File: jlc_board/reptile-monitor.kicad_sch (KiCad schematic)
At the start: 28 parts, among them J1 AudioJack4_SwitchR1, J2 AudioJack4_SwitchR1, J3 PWR CONN, J4 UART, J5 I2C, SW1 RESET, SW2 BOOT, U1 AP2112M-3.3, U2 TCA4307DGKR

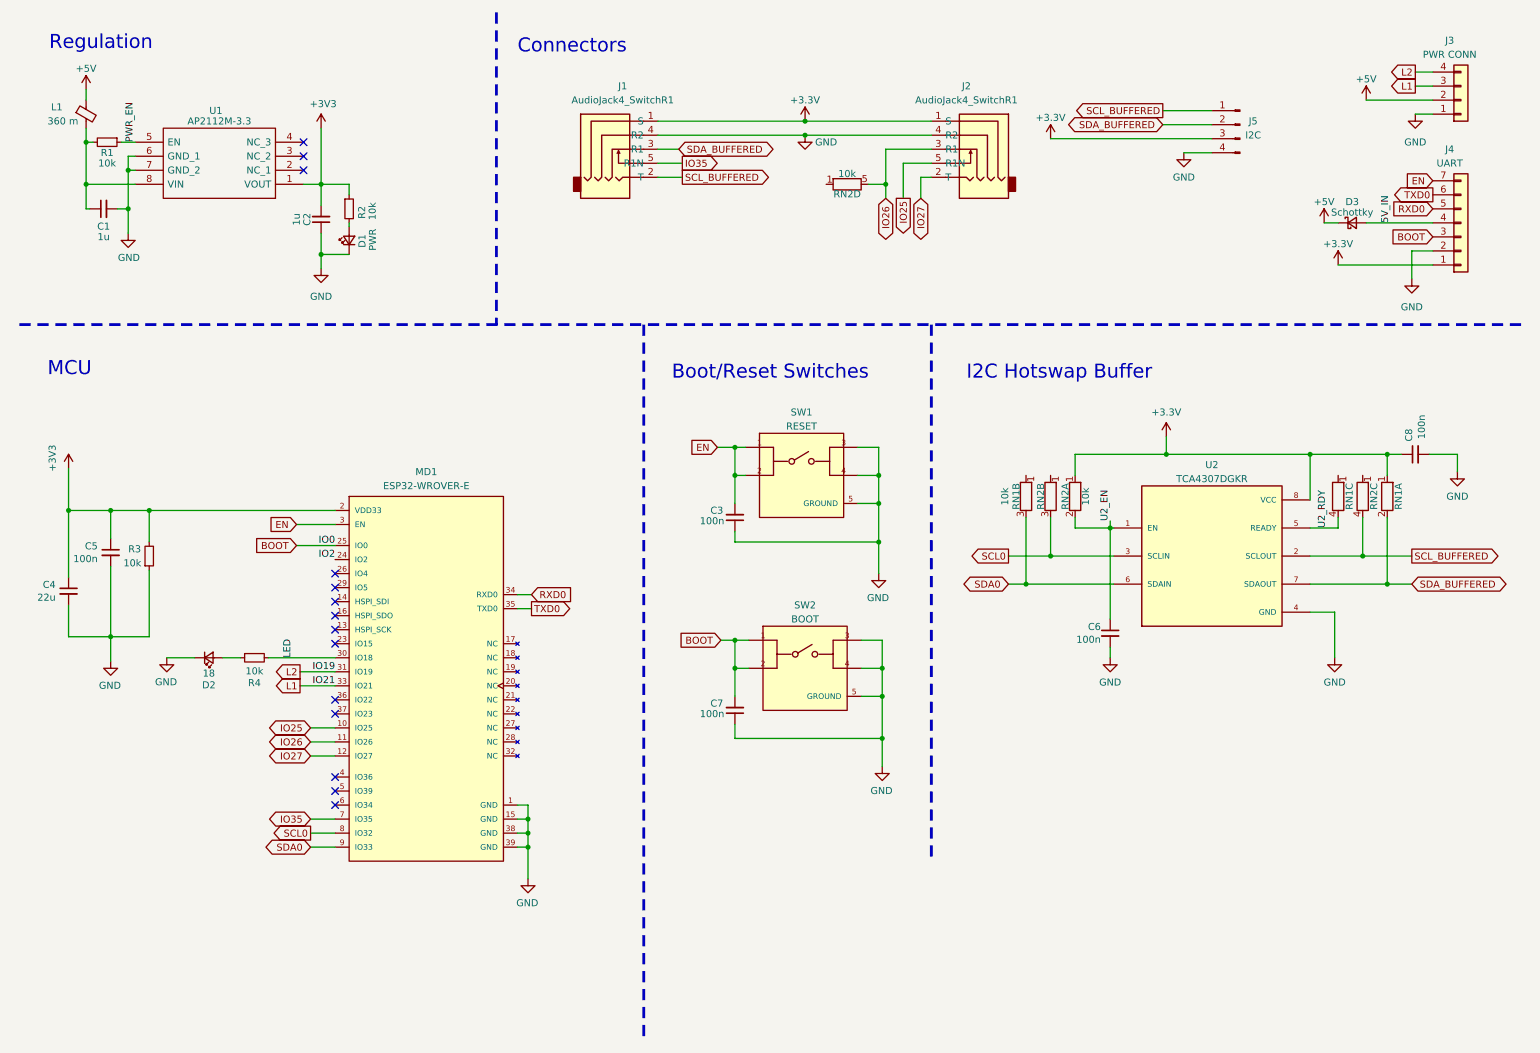
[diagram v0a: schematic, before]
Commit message: v4 reorganization complete
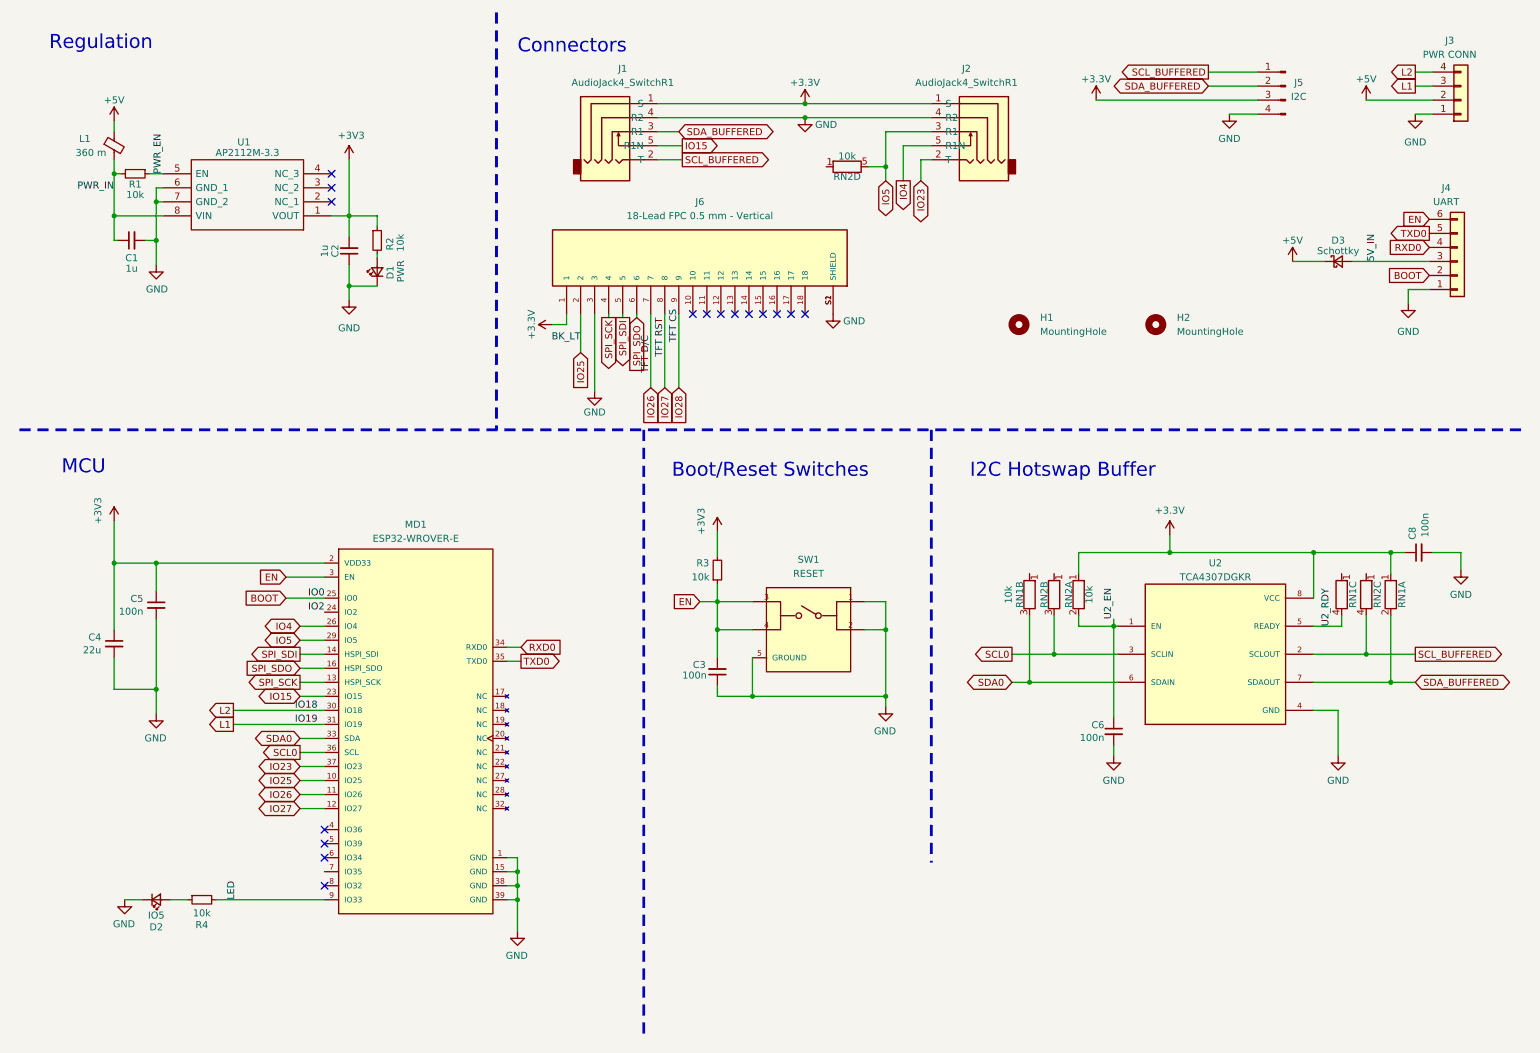
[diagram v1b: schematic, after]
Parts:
- removed C7: 100n, reptile-monitor:C_0603_1608Metric, symbol Device:C_Small
- removed SW2: BOOT, reptile-monitor:CK-KMR221GLFS-MFG, symbol Reptile_Monitor:KMR221GLFS
- added H1, H2: MountingHole, MountingHole:MountingHole_2.2mm_M2_ISO7380, symbol Mechanical:MountingHole
- added J6: 18-Lead FPC 0.5 mm - Vertical, reptile-monitor:TE_1-1734742-8, symbol reptile-monitor:18-Lead FPC 0.5 mm - Vertical
- D2: value 18 -> IO5
- D3: footprint reptile-monitor:D_SOD-523 -> reptile-monitor:D_SMA
- J3: footprint reptile-monitor:PinSocket_1x04_P2.54mm_Vertical -> reptile-monitor:PinSocket_1x04_P2.54mm_Vertical_SMD_Pin1Left
- J4: footprint reptile-monitor:PinHeader_1x07_P2.54mm_Vertical -> reptile-monitor:PinHeader_1x06_P2.54mm_Vertical; symbol Connector_Generic:Conn_01x07 -> Connector_Generic:Conn_01x06
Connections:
- net +3V3: now also J6.1; no longer J4.1 (Pin_1)
- net 5V_IN: now also J4.3 (Pin_3); no longer J4.4 (Pin_4)
- net BOOT: now also J4.2 (Pin_2); no longer J4.3 (Pin_3)
- net EN: now also J4.6 (Pin_6), R3.1, SW1.3, SW1.4; no longer J4.7 (Pin_7), SW1.1, SW1.2
- net GND: now also J4.1 (Pin_1), SW1.1, SW1.2, J6.3, J6.S1 (SHIELD), J6.S2 (SHIELD); no longer J4.2 (Pin_2), R3.1, SW1.3, SW1.4
- net IO25: now also J6.2; no longer J2.5 (R1N)
- net IO26: now also J6.7; no longer J2.3 (R1), RN2.5 (R4.2)
- net IO27: now also J6.8; no longer J2.2 (T)
- net L1: now also MD1.31 (IO19); no longer MD1.33 (IO21)
- net L2: now also MD1.30 (IO18); no longer MD1.31 (IO19)
- net LED: now also MD1.9 (IO33); no longer MD1.30 (IO18)
- net RXD0: now also J4.4 (Pin_4); no longer J4.5 (Pin_5)
- net SCL0: now also MD1.36 (IO22); no longer MD1.8 (IO32)
- net SDA0: now also MD1.33 (IO21); no longer MD1.9 (IO33)
- net TXD0: now also J4.5 (Pin_5); no longer J4.6 (Pin_6)
- net PWR_IN: now reaches C1.1, L1.2, R1.2, U1.8 (VIN)
- net SPI_SCK: now reaches MD1.13 (IO14)
- net SPI_SCK: now also J6.4
- net SPI_SDI: now reaches MD1.14 (IO12)
- net SPI_SDI: now also J6.5
- net SPI_SDO: now reaches MD1.16 (IO13)
- net SPI_SDO: now also J6.6
- net IO15: now reaches MD1.23 (IO15)
- net IO15: now also J1.5 (R1N)
- net IO4: now reaches MD1.26 (IO4)
- net IO4: now also J2.5 (R1N)
- net IO5: now reaches MD1.29 (IO5)
- net IO5: now also J2.3 (R1), RN2.5 (R4.2)
- net IO23: now reaches MD1.37 (IO23)
- net IO23: now also J2.2 (T)
- net IO35: no longer names the net of MD1.7 (IO35)
- net IO35: no longer J1.5 (R1N)
- new net IO28: J6.9
- no-connect marks 14 -> 16
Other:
- moved on the sheet: C1, C2, C3, C4, C5, C6, C8, D1, D2, D3, J1, J2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
